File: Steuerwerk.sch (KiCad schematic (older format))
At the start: 128 parts, among them J1 2PinTerminalBlocktg, J10 2PinTerminalBlocktg, J11 2PinTerminalBlocktg, J12 2PinTerminalBlocktg, J2 2PinTerminalBlocktg, J3 3PinTerminalBlocktg, J4 3PinTerminalBlocktg, J5 2PinTerminalBlocktg, J6 2PinTerminalBlocktg, J7 2PinTerminalBlocktg, J8 2PinTerminalBlocktg, J9 2PinTerminalBlocktg, Q1 Q_PNP_BCE, U1 74ls240, U2 74541, U3 74LS161, U4 74LS138, U5 74LS138, U6 74541, U7 74LS374, U8 74LS374

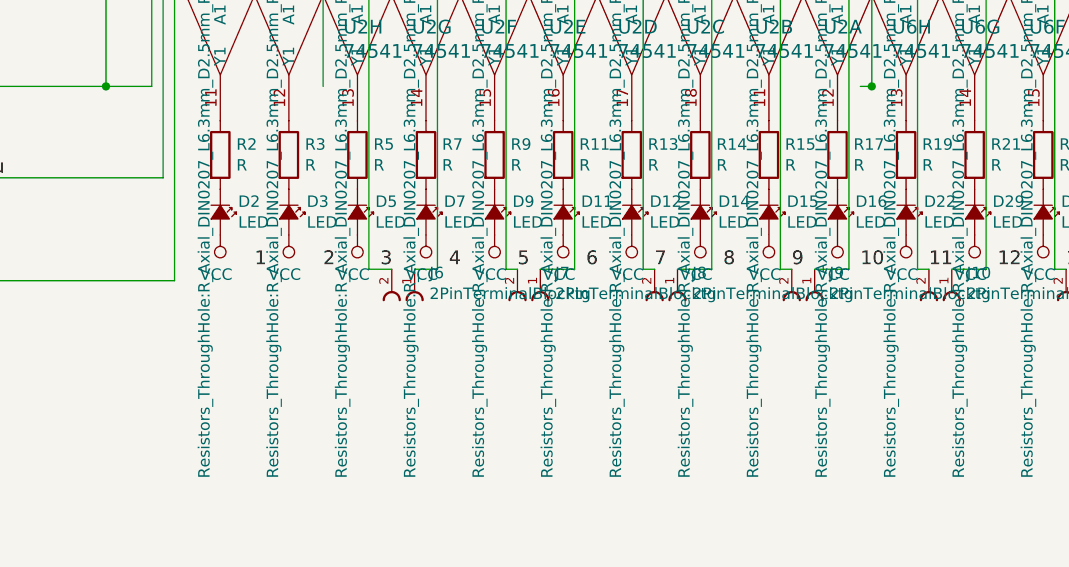
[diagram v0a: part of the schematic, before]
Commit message: Verbindungen zum IC fortgeführt
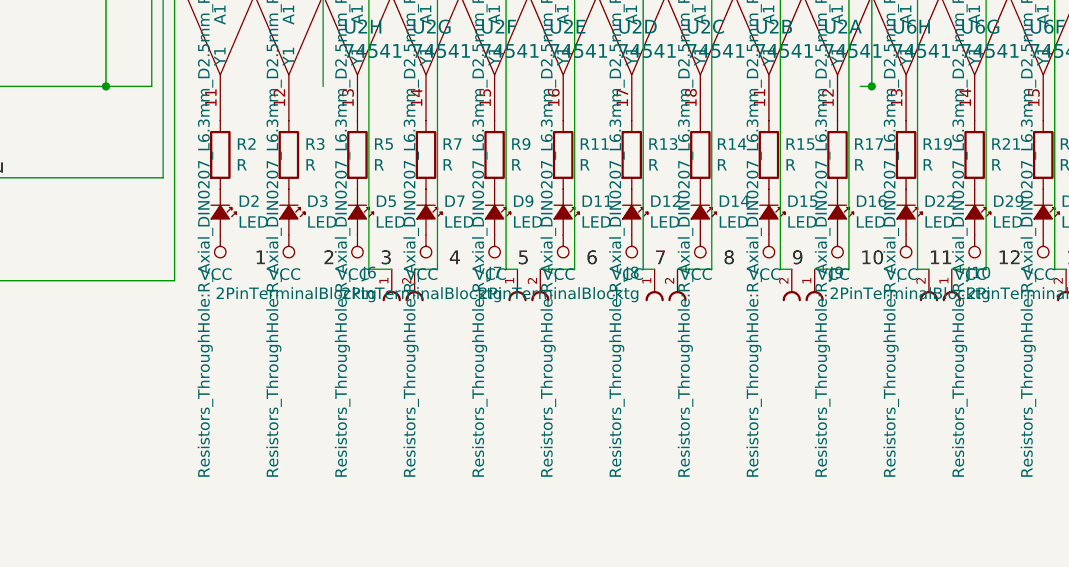
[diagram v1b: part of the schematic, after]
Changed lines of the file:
@@
 L 2PinTerminalBlocktg:2PinTerminalBlocktg J6
 U 1 1 5AC6BD39
-P 2950 7700
-F 0 "J6" V 2766 7765 50  0000 L CNN
-F 1 "2PinTerminalBlocktg" V 2857 7765 50  0000 L CNN
-F 2 "2PinTerminalBlocktg" H 2950 7700 50  0001 L BNN
-F 3 "None" H 2950 7700 50  0001 L BNN
-F 4 "Wurth Electronics" H 2950 7700 50  0001 L BNN "Field4"
-F 5 "None" H 2950 7700 50  0001 L BNN "Field5"
-F 6 "Unavailable" H 2950 7700 50  0001 L BNN "Field6"
-F 7 "TERM BLOCK 2POS HORIZ 5.08MM T/H" H 2950 7700 50  0001 L BNN "Field7"
-F 8 "2PinTerminalBlocktg" H 2950 7700 50  0001 L BNN "Field8"
-	1    2950 7700
-	0    1    1    0
+P 2850 7700
+F 0 "J6" V 2666 7765 50  0000 L CNN
+F 1 "2PinTerminalBlocktg" V 2757 7765 50  0000 L CNN
+F 2 "2PinTerminalBlocktg" H 2850 7700 50  0001 L BNN
+F 3 "None" H 2850 7700 50  0001 L BNN
+F 4 "Wurth Electronics" H 2850 7700 50  0001 L BNN "Field4"
+F 5 "None" H 2850 7700 50  0001 L BNN "Field5"
+F 6 "Unavailable" H 2850 7700 50  0001 L BNN "Field6"
+F 7 "TERM BLOCK 2POS HORIZ 5.08MM T/H" H 2850 7700 50  0001 L BNN "Field7"
+F 8 "2PinTerminalBlocktg" H 2850 7700 50  0001 L BNN "Field8"
+	1    2850 7700
+	0    -1   1    0
 $EndComp
 $Comp
 L 2PinTerminalBlocktg:2PinTerminalBlocktg J7
 U 1 1 5AC6C26F
-P 3500 7700
-F 0 "J7" V 3316 7765 50  0000 L CNN
-F 1 "2PinTerminalBlocktg" V 3407 7765 50  0000 L CNN
-F 2 "2PinTerminalBlocktg" H 3500 7700 50  0001 L BNN
-F 3 "None" H 3500 7700 50  0001 L BNN
-F 4 "Wurth Electronics" H 3500 7700 50  0001 L BNN "Field4"
-F 5 "None" H 3500 7700 50  0001 L BNN "Field5"
-F 6 "Unavailable" H 3500 7700 50  0001 L BNN "Field6"
-F 7 "TERM BLOCK 2POS HORIZ 5.08MM T/H" H 3500 7700 50  0001 L BNN "Field7"
-F 8 "2PinTerminalBlocktg" H 3500 7700 50  0001 L BNN "Field8"
-	1    3500 7700
-	0    1    1    0
+P 3400 7700
+F 0 "J7" V 3216 7765 50  0000 L CNN
+F 1 "2PinTerminalBlocktg" V 3307 7765 50  0000 L CNN
+F 2 "2PinTerminalBlocktg" H 3400 7700 50  0001 L BNN
+F 3 "None" H 3400 7700 50  0001 L BNN
+F 4 "Wurth Electronics" H 3400 7700 50  0001 L BNN "Field4"
+F 5 "None" H 3400 7700 50  0001 L BNN "Field5"
+F 6 "Unavailable" H 3400 7700 50  0001 L BNN "Field6"
+F 7 "TERM BLOCK 2POS HORIZ 5.08MM T/H" H 3400 7700 50  0001 L BNN "Field7"
+F 8 "2PinTerminalBlocktg" H 3400 7700 50  0001 L BNN "Field8"
+	1    3400 7700
+	0    -1   1    0
 $EndComp
 $Comp
 L 2PinTerminalBlocktg:2PinTerminalBlocktg J8
 U 1 1 5AC6C549
-P 4100 7700
-F 0 "J8" V 3916 7765 50  0000 L CNN
-F 1 "2PinTerminalBlocktg" V 4007 7765 50  0000 L CNN
-F 2 "2PinTerminalBlocktg" H 4100 7700 50  0001 L BNN
-F 3 "None" H 4100 7700 50  0001 L BNN
-F 4 "Wurth Electronics" H 4100 7700 50  0001 L BNN "Field4"
-F 5 "None" H 4100 7700 50  0001 L BNN "Field5"
-F 6 "Unavailable" H 4100 7700 50  0001 L BNN "Field6"
-F 7 "TERM BLOCK 2POS HORIZ 5.08MM T/H" H 4100 7700 50  0001 L BNN "Field7"
-F 8 "2PinTerminalBlocktg" H 4100 7700 50  0001 L BNN "Field8"
-	1    4100 7700
-	0    1    1    0
+P 4000 7700
+F 0 "J8" V 3816 7765 50  0000 L CNN
+F 1 "2PinTerminalBlocktg" V 3907 7765 50  0000 L CNN
+F 2 "2PinTerminalBlocktg" H 4000 7700 50  0001 L BNN
+F 3 "None" H 4000 7700 50  0001 L BNN
+F 4 "Wurth Electronics" H 4000 7700 50  0001 L BNN "Field4"
+F 5 "None" H 4000 7700 50  0001 L BNN "Field5"
+F 6 "Unavailable" H 4000 7700 50  0001 L BNN "Field6"
+F 7 "TERM BLOCK 2POS HORIZ 5.08MM T/H" H 4000 7700 50  0001 L BNN "Field7"
+F 8 "2PinTerminalBlocktg" H 4000 7700 50  0001 L BNN "Field8"
+	1    4000 7700
+	0    -1   1    0
 $EndComp
 $Comp
@@
 	3400 7500 3350 7500
 Wire Wire Line
-	3050 7500 2950 7500
-Wire Wire Line
 	2850 7500 2750 7500
 Connection ~ 7800 1350
@@
 Wire Wire Line
 	7550 1000 7550 1150
+Wire Wire Line
+	3050 7500 2950 7500
 $EndSCHEMATC
